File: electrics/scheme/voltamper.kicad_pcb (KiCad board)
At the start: 2 copper layers, 136 parts, among them K1 swd, K2 servo-1, K3 servo-2, P1 boot, P2 boot, P3 -, P4 +, P5 work, P6 aux, P7 ref, Q1 bc857, Q2 bc847, Q3 bc857, Q4 bc847, Q5 irlml2244, Q6 bc847, Q7 bc847, Q8 bc847, SW1 btn-1, SW2 btn-2, U1 CRYSTAL-4PIN, U10 TDA2030A, U11 INA126, U12 SPARTAN-SIP-9007, U2 CP2102, U3 MICRO-USB-B, U4 MCP1703T-3302E/CB, U5 MCP1703T-3302E/CB, U6 NCP3063, U7 SPARTAN-SIP-9007, U8 NCP3063, U9 SPARTAN-SIP-9007

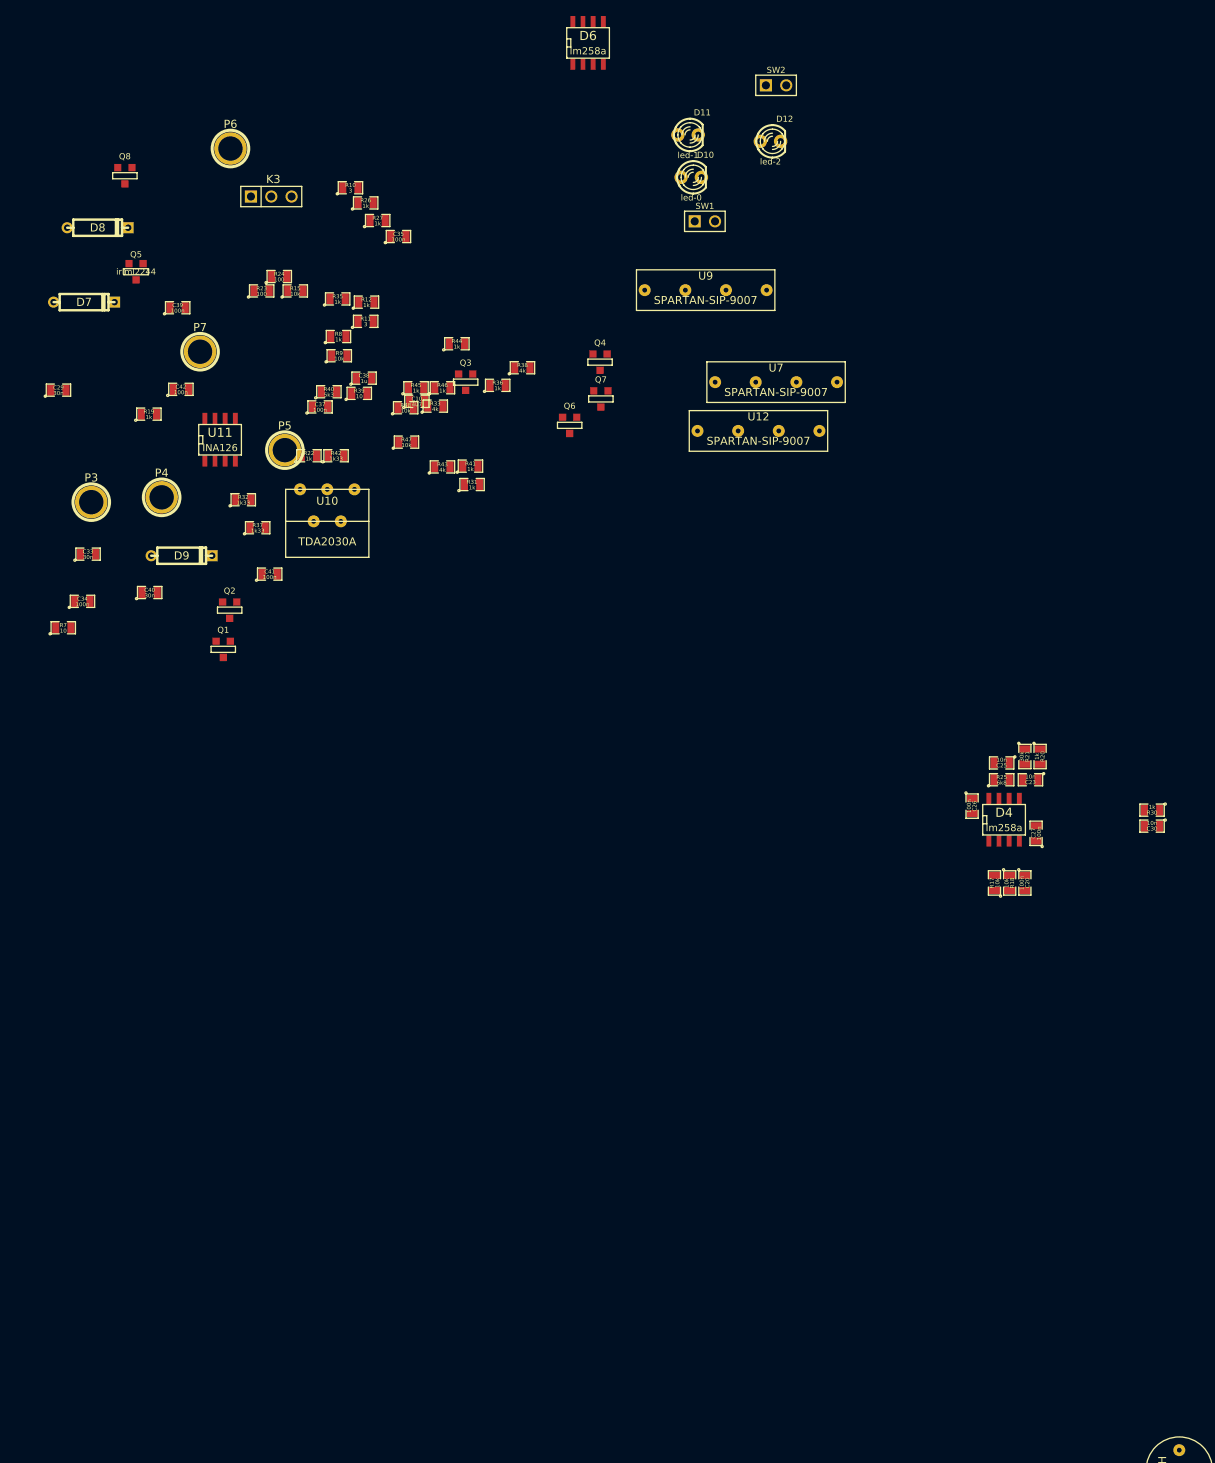
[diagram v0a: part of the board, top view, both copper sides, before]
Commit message: a
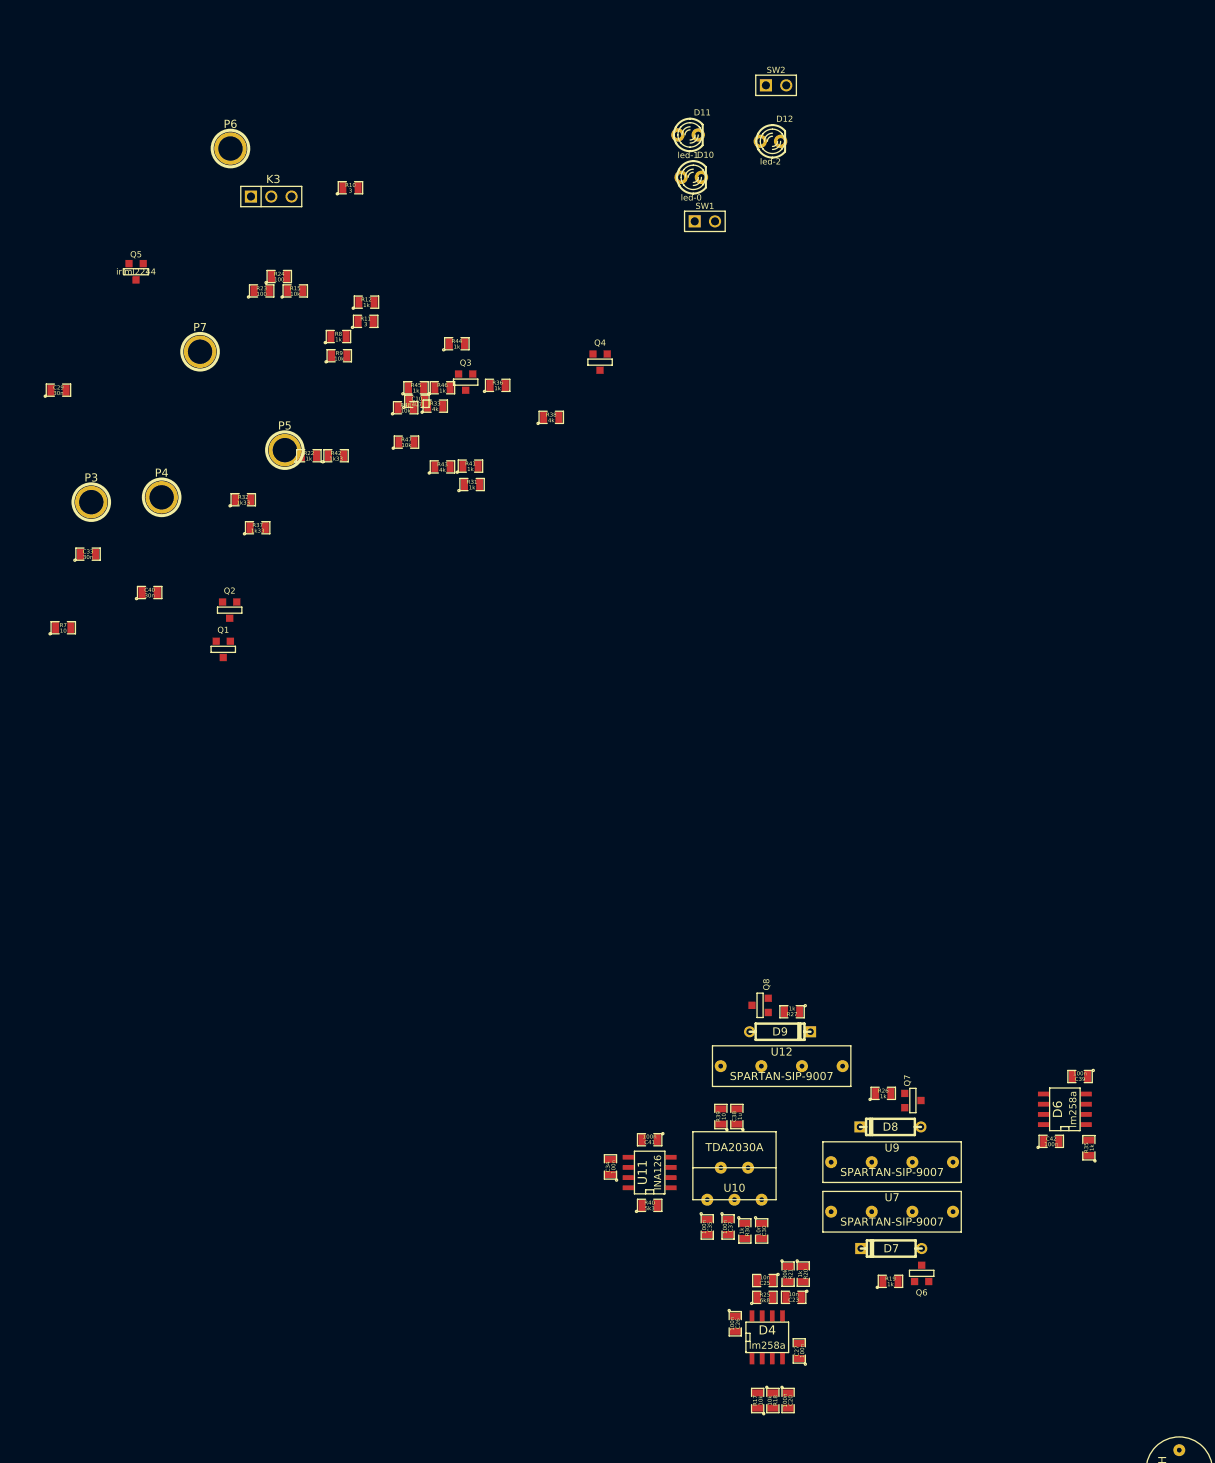
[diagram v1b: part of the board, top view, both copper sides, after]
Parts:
- moved D7 155.5 mm to (59.3, 105.9), turned to 180 degrees
- moved D8 149.8 mm to (59.2, 90.7), turned to 180 degrees
- moved C39 148.2 mm to (82.9, 84.4), turned to 180 degrees
- moved D6 146.0 mm to (81.0, 88.5), turned to 90 degrees
- moved C42 143.8 mm to (79.3, 92.5)
- moved R19 142.6 mm to (59.2, 110.0)
- moved R35 141.7 mm to (84.0, 93.3), turned to 90 degrees
- moved Q8 130.6 mm to (42.9, 75.5), turned to 270 degrees
- moved C35 129.7 mm to (36.3, 103.2), turned to 270 degrees
- moved R26 128.7 mm to (58.3, 86.5)
- moved Q6 114.8 mm to (63.1, 109.0), turned to 180 degrees
- moved C37 114.5 mm to (38.9, 103.2), turned to 270 degrees
- moved R27 111.6 mm to (46.9, 76.3), turned to 180 degrees
- moved U9 111.5 mm to (59.4, 95.1)
- moved R40 109.3 mm to (29.1, 100.5)
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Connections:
- C22 pad 1: /aux-2 -> /v+
- C24 pad 1: /aux-2 -> /v+
- C26 pad 1: /aux-2 -> /v+
- C34 pad 1: /aux-2 -> /v+
- C35 pad 1: /aux-2 -> /v+
- C42 pad 1: /aux-2 -> /v+
- D3 pad 2: /aux-2 -> /v+
- D4 pad 8: /aux-2 -> /v+
- D6 pad 8: /aux-2 -> /v+
- D7 pad 2: /aux-2 -> /v+
- D8 pad 2: /aux-2 -> /v+
- D9 pad 2: /aux-2 -> /v+
- R16 pad 2: /aux-2 -> /v+
- U10 pad 5: /aux-2 -> /v+
- U11 pad 7: /aux-2 -> /v+
- U12 pad 3: /aux-2 -> /v+
- U7 pad 2: /aux-2 -> /v+
- U9 pad 2: /curr-1 -> /v+
- U9 pad 3: /aux-2 -> /curr-1
